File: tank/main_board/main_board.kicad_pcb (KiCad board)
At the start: 2 copper layers, 70.3 x 55.2 mm, 43 parts, among them J1 PowerIn, J10 Bump1, J11 Programming Header, J12 SigOut, J13 Encoder0, J14 Encoder1, J16 PowerOut, J2 M1, J20 PowerMotor, J3 M2, J4 LEDs, J5 M0, J6 Spk, J7 Hall2, J8 Hall1, J9 Bump0, Q1 2N3904, U1 L7805, U2 ATMEGA328P-PU, U3 SN74HC595, U4 TB6612FNG, U5 TB6612FNG, Y1 Crystal

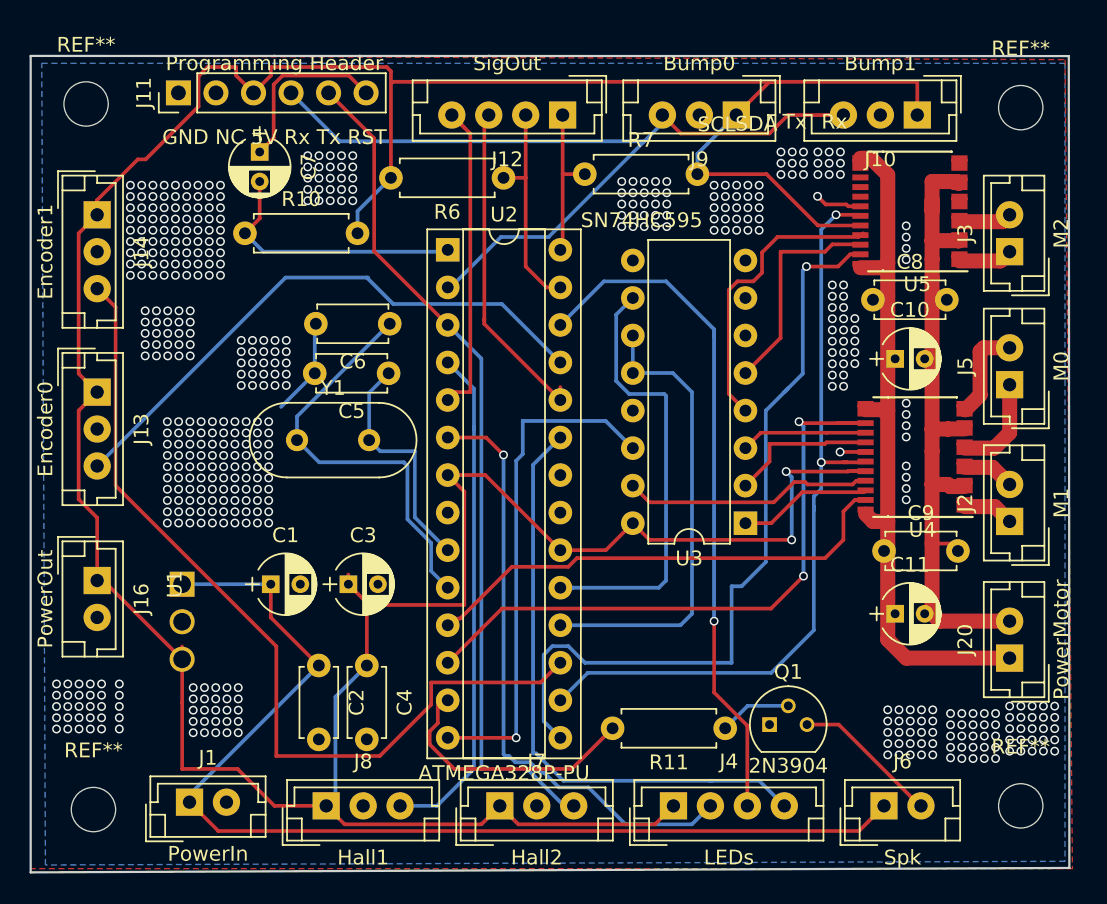
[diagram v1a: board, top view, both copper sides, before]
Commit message: main board 0.8 WIP
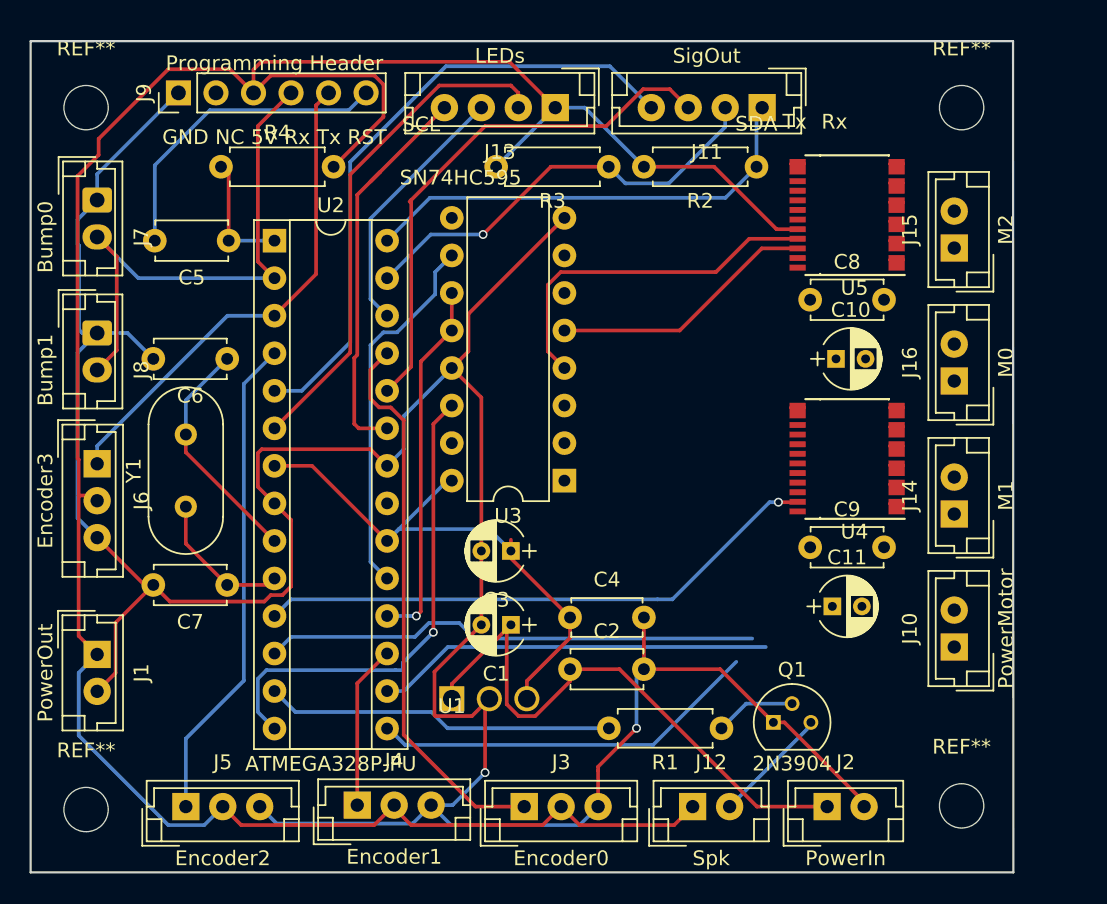
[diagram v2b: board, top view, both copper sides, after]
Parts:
- removed the REF** at (101.2, 77.8)
- removed the REF** at (101.8, 125.5)
- added REF**: MountingHole_3mm, MountingHole:MountingHole_3mm, F.Cu at (101.2, 125.5)
- added REF**: MountingHole_3mm, MountingHole:MountingHole_3mm, F.Cu at (101.2, 78.0)
- C2, C6, C8, C9: footprint Capacitors_THT:C_Disc_D4.7mm_W2.5mm_P5.00mm -> Capacitor_THT:C_Disc_D4.7mm_W2.5mm_P5.00mm
- C5: value C5 -> C_Small; footprint Capacitors_THT:C_Disc_D4.7mm_W2.5mm_P5.00mm -> Capacitor_THT:C_Disc_D4.7mm_W2.5mm_P5.00mm
- C7: value CP -> C7; footprint Capacitors_THT:CP_Radial_D4.0mm_P2.00mm -> Capacitor_THT:C_Disc_D4.7mm_W2.5mm_P5.00mm
- J5: renamed from J8; value Hall1 -> Encoder2
- J6: renamed from J7; value Hall2 -> Encoder3
- J7: renamed from J9; footprint JST:JST_EH_B03B-EH-A_03x2.50mm_Straight -> Connector_JST:JST_EH_B2B-EH-A_1x02_P2.50mm_Vertical
- J8: renamed from J10; footprint JST:JST_EH_B03B-EH-A_03x2.50mm_Straight -> Connector_JST:JST_EH_B2B-EH-A_1x02_P2.50mm_Vertical
- moved J8 57.4 mm to (102.0, 93.2), turned to 270 degrees
- moved J13 47.9 mm to (133.0, 78.0), turned to 180 degrees
- moved J4 43.7 mm to (119.6, 125.2), turned to 0 degrees
- moved J7 43.6 mm to (102.0, 84.2), turned to 270 degrees
- moved J2 43.2 mm to (151.4, 125.3)
- moved J3 40.3 mm to (130.9, 125.3), turned to 0 degrees
- moved J6 35.8 mm to (102.0, 102.1), turned to 270 degrees
- moved C7 29.4 mm to (110.8, 110.3), turned to 180 degrees
- moved U1 19.8 mm to (126.0, 118.0), turned to 0 degrees
- moved C2 17.0 mm to (134.0, 116.0), turned to 0 degrees
- moved C1 16.5 mm to (130.0, 113.0), turned to 180 degrees
- moved C4 14.1 mm to (134.0, 112.5), turned to 0 degrees
- moved C5 14.1 mm to (110.9, 87.0)
- moved J11 13.5 mm to (147.0, 78.0)
- moved J12 13.0 mm to (142.3, 125.3)
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- renumbered J16 to J1, J20 to J10, J12 to J11, J6 to J12, J4 to J13, J2 to J14, J3 to J15, J5 to J16, J1 to J2, J13 to J3, J14 to J4, J11 to J9, R11 to R1, R7 to R2, R6 to R3, R10 to R4
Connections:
- C5 pad 2: GND -> Net-(C5-Pad2)
- C7 pad 2: Net-(C7-Pad2) -> GND
- J12 pad 1: 9V -> 4.5V
- J3 pad 1: 4.5V -> Encoder0
- J3 pad 2: GND -> 4.5V
- J3 pad 3: Encoder0 -> GND
- J4 pad 1: 4.5V -> Encoder1
- J4 pad 2: GND -> 4.5V
- J4 pad 3: Encoder1 -> GND
- J5 pad 1: 4.5V -> Encoder2
- J5 pad 2: GND -> 4.5V
- J5 pad 3: TurretEncoder -> GND
- J6 pad 1: 4.5V -> Encoder3
- J6 pad 2: GND -> 4.5V
- J6 pad 3: TurretCal -> GND
- J7 pad 1: 4.5V -> GND
- J7 pad 2: GND -> Bump
- J8 pad 1: 4.5V -> GND
- J8 pad 2: GND -> Bump
- J9 pad 5: TurretCal -> Encoder3
- J9 pad 6: Net-(C7-Pad1) -> Net-(C5-Pad2)
- R4 pad 1: Net-(C7-Pad2) -> Net-(C5-Pad1)
- U2 pad 1: Net-(C7-Pad2) -> Net-(C5-Pad1)
- U2 pad 10: Net-(C6-Pad1) -> Net-(C7-Pad1)
- U2 pad 3: TurretCal -> Encoder3
- U2 pad 4: TurretEncoder -> Encoder2
- U2 pad 9: Net-(C5-Pad1) -> Net-(C6-Pad1)
- Y1 pad 1: Net-(C6-Pad1) -> Net-(C7-Pad1)
- Y1 pad 2: Net-(C5-Pad1) -> Net-(C6-Pad1)
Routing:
- net GND: track 64.3 -> 202.5 mm, vias 468 -> 2
- net TurretCal: track 57.3 -> 0.00 mm
- net Vm: track 48.9 -> 0.00 mm
- net Encoder1: track 59.4 -> 11.1 mm
- net 4.5V: track 249.2 -> 207.9 mm, vias 2 -> 0
- net 9V: track 74.6 -> 39.8 mm
- net TurretEncoder: track 34.5 -> 0.00 mm
- net Encoder3: track 0.00 -> 33.4 mm
- net Encoder2: track 0.00 -> 33.2 mm
- net LED1: track 47.8 -> 17.7 mm, vias 1 -> 0
- net M2PWM: track 53.3 -> 26.4 mm, vias 1 -> 0
- net MEnable: track 53.1 -> 27.2 mm, vias 2 -> 0
- net Net-(C5-Pad2): track 0.00 -> 21.4 mm
- net Bump: track 58.2 -> 37.2 mm
- net IRRx: track 22.2 -> 42.9 mm
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- removed copper zone on B.Cu, net GND
- removed copper zone on F.Cu, net GND
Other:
- board size 70.3 x 55.2 mm -> 66.5 x 56.2 mm
